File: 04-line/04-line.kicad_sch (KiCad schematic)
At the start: 84 parts, among them J2 VL53L0X, J2 WRITER CONN, J3 ToMAIN, U24 STM32F446RETx

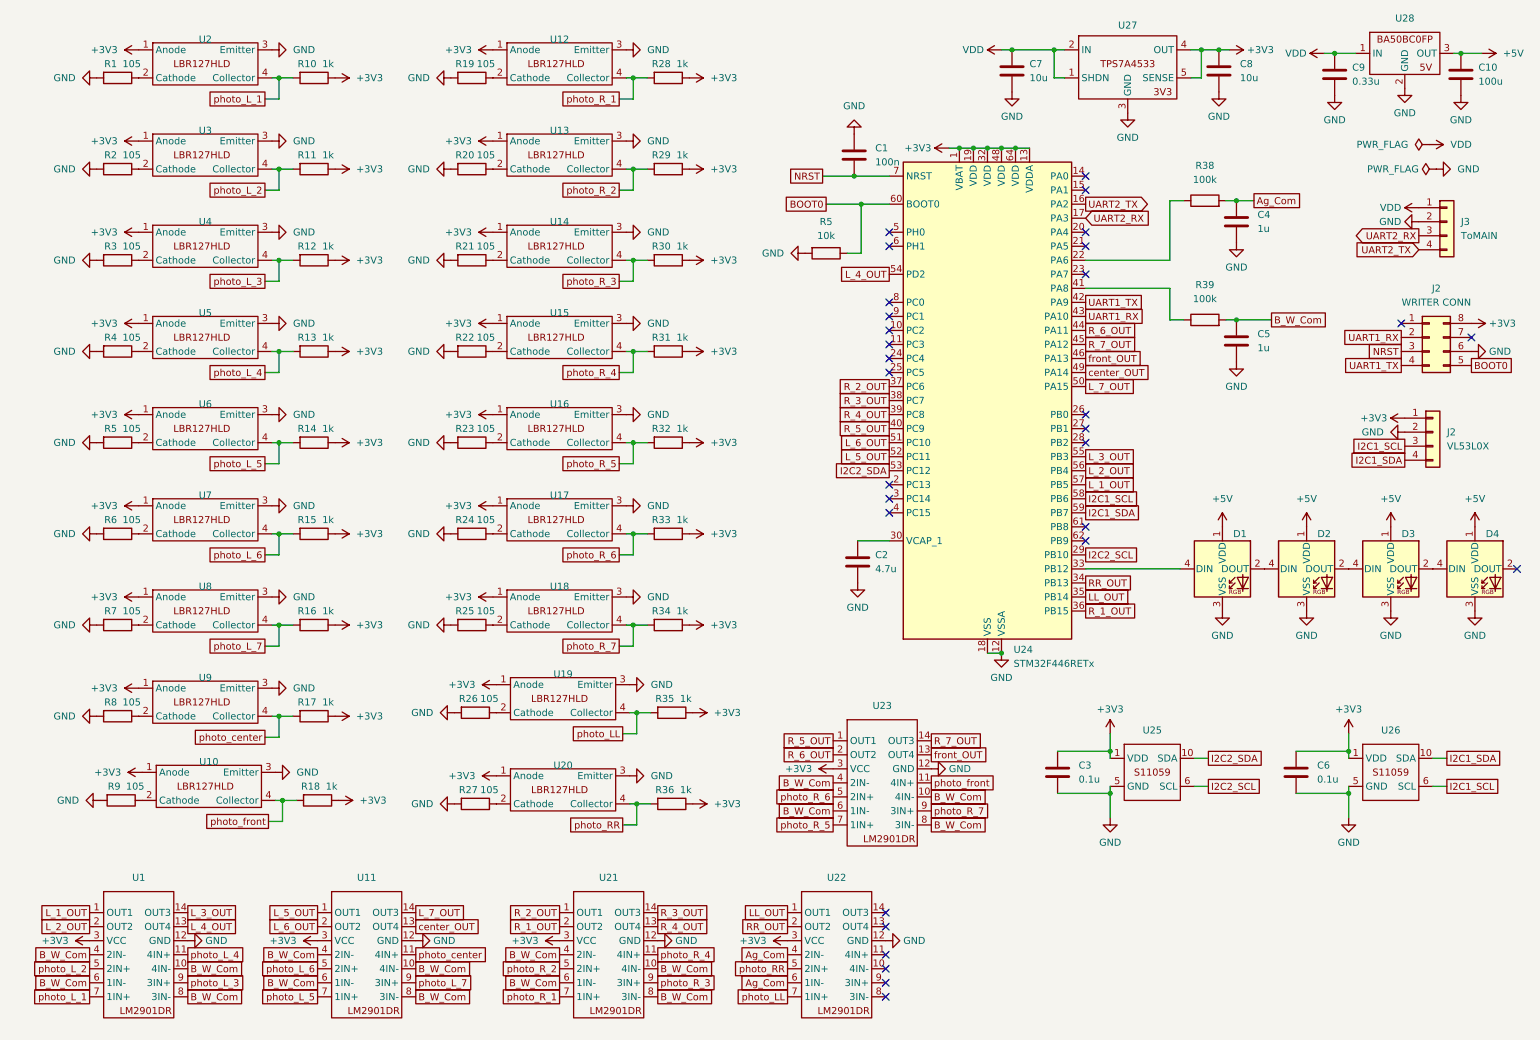
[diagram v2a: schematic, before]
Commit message: ラインセンサ完成
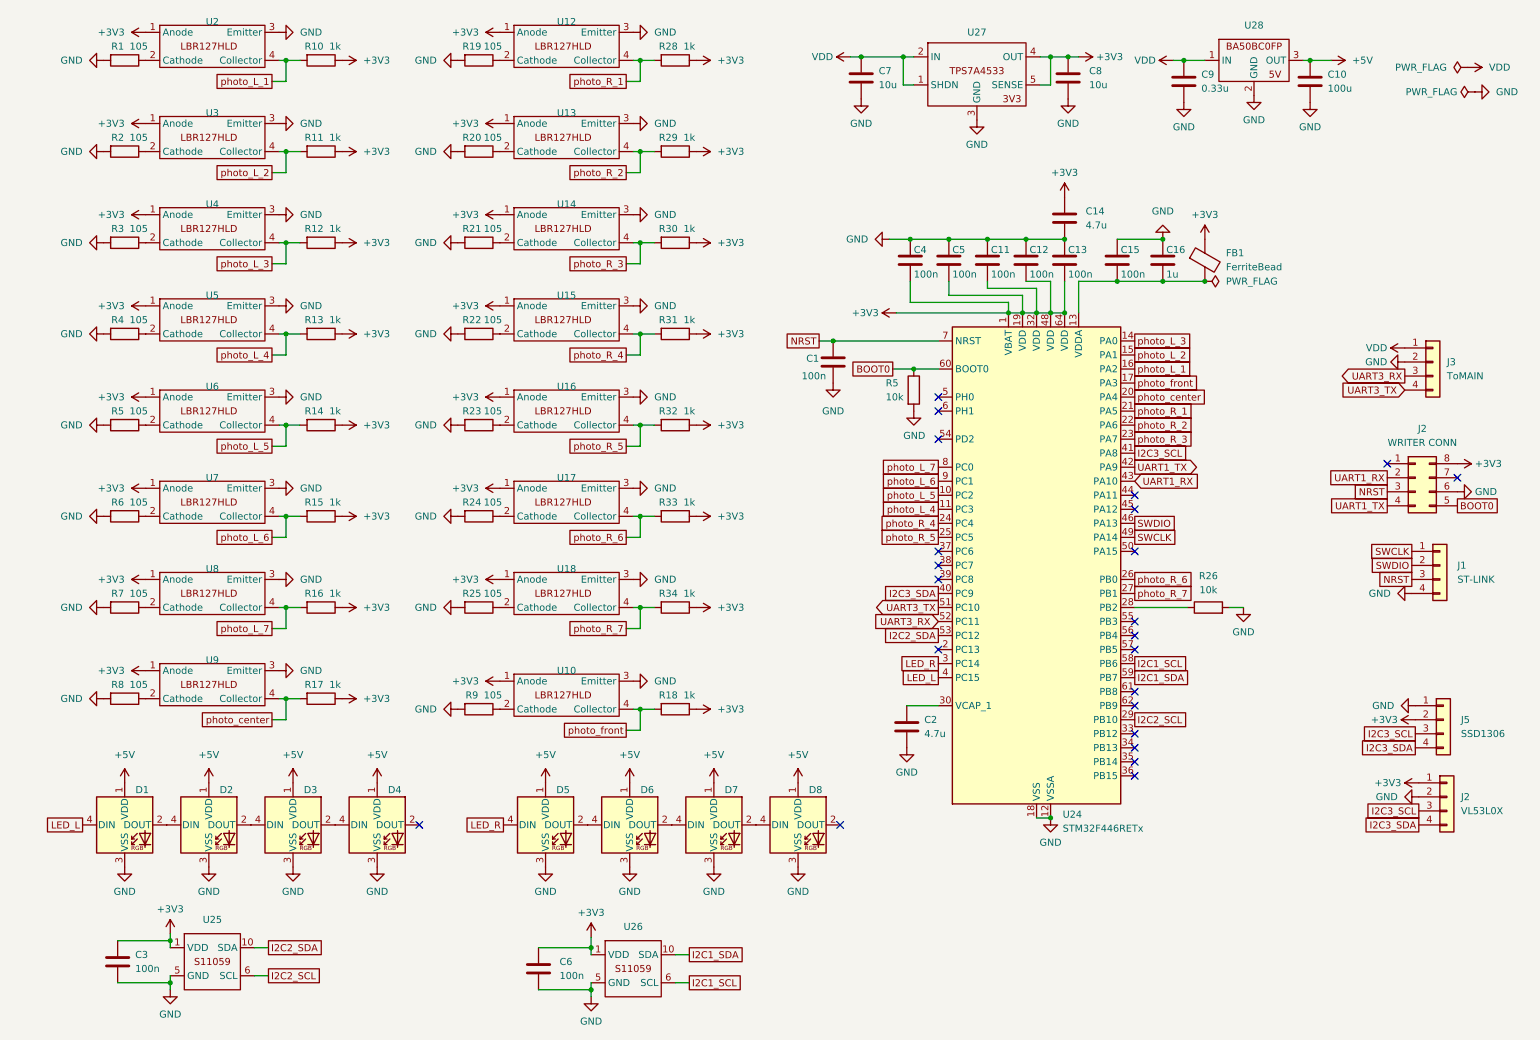
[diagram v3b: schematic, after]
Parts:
- removed R27: 105, Resistor_SMD:R_0603_1608Metric, symbol Device:R
- removed R35, R36: 1k, Resistor_SMD:R_1206_3216Metric, symbol Device:R
- removed R38, R39: 100k, Resistor_SMD:R_0805_2012Metric, symbol Device:R
- removed U1, U11, U21, U22, U23: ~, Package_SO:SOIC-14_3.9x8.7mm_P1.27mm, symbol JLCPCB_items:LM2901DR
- removed U19, U20: ~, Akiduki:LBR127HLD, symbol akiduki:LBR127HLD
- added C11, C12, C13, C15: 100n, Capacitor_SMD:C_0402_1005Metric, symbol Device:C
- added C14: 4.7u, Capacitor_SMD:C_0402_1005Metric, symbol Device:C
- added C16: 1u, Capacitor_SMD:C_0402_1005Metric, symbol Device:C
- added D5, D6, D7, D8: WS2812B, LED_SMD:LED_WS2812B_PLCC4_5.0x5.0mm_P3.2mm, symbol LED:WS2812B
- added FB1: FerriteBead, Resistor_SMD:R_0805_2012Metric, symbol Device:FerriteBead
- added J1: ST-LINK, Connector_PinHeader_2.54mm:PinHeader_1x04_P2.54mm_Vertical, symbol Connector_Generic:Conn_01x04
- added J5: SSD1306, Connector_PinHeader_2.54mm:PinHeader_1x04_P2.54mm_Vertical, symbol Connector_Generic:Conn_01x04
- C1: footprint Capacitor_SMD:C_0805_2012Metric -> Capacitor_SMD:C_0402_1005Metric; LCSC (none) -> C1525
- C10: footprint Capacitor_SMD:C_0805_2012Metric -> Capacitor_SMD:C_1206_3216Metric; LCSC (none) -> C7432784
- C2: footprint Capacitor_SMD:C_0805_2012Metric -> Capacitor_SMD:C_0402_1005Metric; LCSC (none) -> C23733
- C3, C6: value 0.1u -> 100n; footprint Capacitor_SMD:C_0805_2012Metric -> Capacitor_SMD:C_0402_1005Metric; LCSC (none) -> C1525
- C4, C5: value 1u -> 100n; footprint Capacitor_SMD:C_0805_2012Metric -> Capacitor_SMD:C_0402_1005Metric; LCSC (none) -> C1525
- C7, C8: footprint Capacitor_SMD:C_0805_2012Metric -> Capacitor_SMD:C_0603_1608Metric; LCSC (none) -> C19702
- C9: LCSC (none) -> C2961026
- D1, D2, D3, D4: LCSC (none) -> C2843785
- R26: value 105 -> 10k; LCSC C128061 -> C137819
- R5: footprint Resistor_SMD:R_0805_2012Metric -> Resistor_SMD:R_0603_1608Metric; LCSC C17414 -> C137819
- U24: LCSC (none) -> C69336
- U27: LCSC (none) -> C2877942
- U28: LCSC (none) -> C2909275
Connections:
- net Ag_Com is gone; now on net GND: C4.1
- net B_W_Com is gone; now on net GND: C5.1
- net +3V3: now also C4.2, C5.2, C11.2, C12.2, C13.2, C14.1, FB1.1, J5.2 (Pin_2); no longer U24.13 (VDDA)
- net +5V: now also D5.1 (VDD), D6.1 (VDD), D7.1 (VDD), D8.1 (VDD)
- net GND: now also C11.1, C12.1, C13.1, C14.2, C15.1, C16.1, D5.3 (VSS), D6.3 (VSS), D7.3 (VSS), D8.3 (VSS), J1.4 (Pin_4), J5.1 (Pin_1); no longer C4.2, C5.2
- net I2C1_SCL: no longer J2.3 (Pin_3)
- net I2C1_SDA: no longer J2.4 (Pin_4)
- net NRST: now also J1.3 (Pin_3)
- net photo_L_1: now also U24.16 (PA2)
- net photo_L_2: now also U24.15 (PA1)
- net photo_L_3: now also U24.14 (PA0)
- net photo_L_4: now also U24.11 (PC3)
- net photo_L_5: now also U24.10 (PC2)
- net photo_L_6: now also U24.9 (PC1)
- net photo_L_7: now also U24.8 (PC0)
- net photo_R_1: now also U24.21 (PA5)
- net photo_R_2: now also U24.22 (PA6)
- net photo_R_3: now also U24.23 (PA7)
- net photo_R_4: now also U24.24 (PC4)
- net photo_R_5: now also U24.25 (PC5)
- net photo_R_6: now also U24.26 (PB0)
- net photo_R_7: now also U24.27 (PB1)
- net photo_center: now also U24.20 (PA4)
- net photo_front: now also U24.17 (PA3)
- net at R26.1: now also U24.28 (PB2)
- net at U24.33 (PB12): no longer D1.4 (DIN)
- net I2C3_SCL: now reaches U24.41 (PA8)
- net I2C3_SCL: now also J2.3 (Pin_3), J5.3 (Pin_3)
- net LED_R: now reaches U24.3 (PC14)
- net LED_R: now also D5.4 (DIN)
- net LED_L: now reaches U24.4 (PC15)
- net LED_L: now also D1.4 (DIN)
- net LL_OUT: no longer names the net of U24.35 (PB14)
- net L_1_OUT: no longer names the net of U24.57 (PB5)
- net L_2_OUT: no longer names the net of U24.56 (PB4)
- net L_3_OUT: no longer names the net of U24.55 (PB3)
- net L_4_OUT: no longer names the net of U24.54 (PD2)
- net L_5_OUT renamed UART3_RX
- net UART3_RX: now also J3.3 (Pin_3)
- net L_6_OUT renamed UART3_TX
- net UART3_TX: now also J3.4 (Pin_4)
- net L_7_OUT: no longer names the net of U24.50 (PA15)
- net RR_OUT: no longer names the net of U24.34 (PB13)
- net R_1_OUT: no longer names the net of U24.36 (PB15)
- net R_2_OUT: no longer names the net of U24.37 (PC6)
- net R_3_OUT: no longer names the net of U24.38 (PC7)
- net R_4_OUT: no longer names the net of U24.39 (PC8)
- net R_5_OUT renamed I2C3_SDA
- net I2C3_SDA: now also J2.4 (Pin_4), J5.4 (Pin_4)
- net R_6_OUT: no longer names the net of U24.44 (PA11)
- net R_7_OUT: no longer names the net of U24.45 (PA12)
- removed net UART2_RX: J3.3 (Pin_3), U24.17 (PA3)
- removed net UART2_TX: J3.4 (Pin_4), U24.16 (PA2)
- net center_OUT renamed SWCLK
- net SWCLK: now also J1.1 (Pin_1)
- net front_OUT renamed SWDIO
- net SWDIO: now also J1.2 (Pin_2)
- new net: C15.2, C16.2, FB1.2, U24.13 (VDDA)
- new net: D5.2 (DOUT), D6.4 (DIN)
- new net: D6.2 (DOUT), D7.4 (DIN)
- new net: D7.2 (DOUT), D8.4 (DIN)
- no-connect marks 30 -> 23
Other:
- company: (none) -> tuton
- moved on the sheet: C1, C10, C2, C3, C6, C7, C8, C9, D1, D2, D3, D4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
